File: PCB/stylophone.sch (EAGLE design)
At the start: 24 parts, among them IC2 LM358N

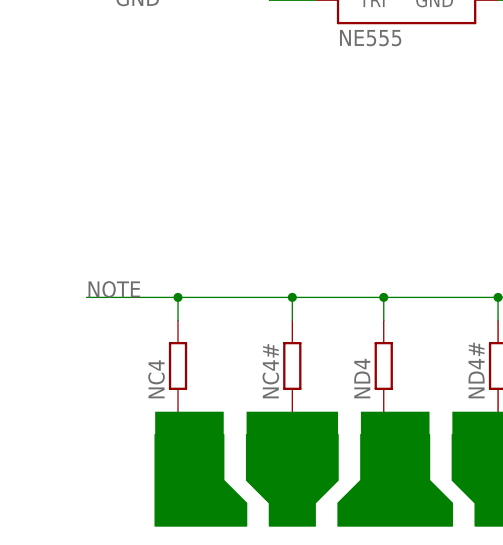
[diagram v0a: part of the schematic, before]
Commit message: almost done
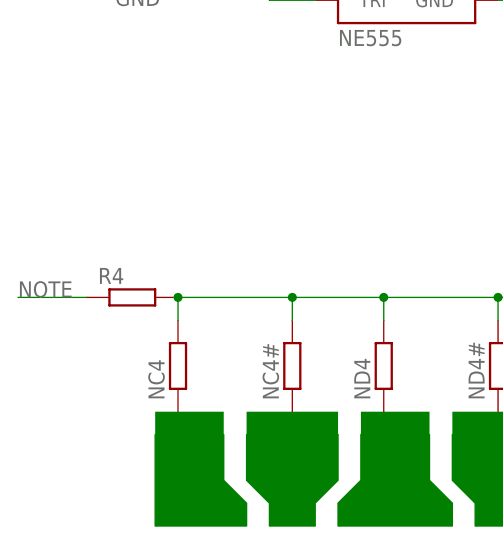
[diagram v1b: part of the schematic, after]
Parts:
- added R4: (no value), rcl:R-EU_0204/5
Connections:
- new net KEYBOARD: NA4#.2, NA4.2, NB4.2, NC4#.2, NC4.2, ND4#.2, ND4.2, NE4.2, NF4#.2, NF4.2, NG4#.2, NG4.2, R4.2
- net NOTE: now also R4.1; no longer NA4#.2, NA4.2, NB4.2, NC4#.2, NC4.2, ND4#.2, ND4.2, NE4.2, NF4#.2, NF4.2, NG4#.2, NG4.2
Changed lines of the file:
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@@
 <part name="R8" library="resistor" deviceset="R-TRIMM" device="5X"/>
 <part name="SV2" library="con-lstb" deviceset="MA05-1" device=""/>
+<part name="R4" library="rcl" deviceset="R-EU_" device="0204/5"/>
 </parts>
 <sheets>
@@
 <instance part="R8" gate="G$1" x="142.24" y="127"/>
 <instance part="SV2" gate="G$1" x="226.06" y="127" rot="R180"/>
+<instance part="R4" gate="G$1" x="25.4" y="86.36"/>
 </instances>
 <busses>
@@
 </segment>
 <segment>
+<pinref part="R4" gate="G$1" pin="1"/>
+<wire x1="20.32" y1="86.36" x2="12.7" y2="86.36" width="0.1524" layer="91"/>
+<label x="12.7" y="86.36" size="1.778" layer="95"/>
+</segment>
+</net>
+<net name="N$1" class="0">
+<segment>
+<pinref part="VIBRATO" gate="G$1" pin="CON"/>
+<wire x1="134.62" y1="121.92" x2="137.16" y2="121.92" width="0.1524" layer="91"/>
+<pinref part="C4" gate="G$1" pin="1"/>
+<wire x1="137.16" y1="121.92" x2="139.7" y2="119.38" width="0.1524" layer="91"/>
+</segment>
+</net>
+<net name="N$3" class="0">
+<segment>
+<pinref part="R7" gate="G$1" pin="1"/>
+<pinref part="R3" gate="G$1" pin="2"/>
+<wire x1="111.76" y1="144.78" x2="119.38" y2="144.78" width="0.1524" layer="91"/>
+<pinref part="VIBRATO" gate="G$1" pin="DIS"/>
+<wire x1="114.3" y1="127" x2="111.76" y2="127" width="0.1524" layer="91"/>
+<wire x1="111.76" y1="127" x2="111.76" y2="144.78" width="0.1524" layer="91"/>
+<junction x="111.76" y="144.78"/>
+</segment>
+</net>
+<net name="NOTSTYLUS" class="0">
+<segment>
+<pinref part="VIBRATO" gate="G$1" pin="TRI"/>
+<wire x1="114.3" y1="119.38" x2="109.22" y2="119.38" width="0.1524" layer="91"/>
+<wire x1="109.22" y1="119.38" x2="109.22" y2="134.62" width="0.1524" layer="91"/>
+<pinref part="VIBRATO" gate="G$1" pin="TRE"/>
+<wire x1="109.22" y1="134.62" x2="114.3" y2="134.62" width="0.1524" layer="91"/>
+<pinref part="C3" gate="G$1" pin="1"/>
+<wire x1="109.22" y1="134.62" x2="101.6" y2="134.62" width="0.1524" layer="91"/>
+<junction x="109.22" y="134.62"/>
+<pinref part="R7" gate="G$1" pin="2"/>
+<wire x1="101.6" y1="134.62" x2="99.06" y2="134.62" width="0.1524" layer="91"/>
+<wire x1="101.6" y1="144.78" x2="101.6" y2="134.62" width="0.1524" layer="91"/>
+<junction x="101.6" y="134.62"/>
+</segment>
+</net>
+<net name="N$2" class="0">
+<segment>
+<pinref part="VIBRATO" gate="G$1" pin="OUT"/>
+<wire x1="134.62" y1="127" x2="139.7" y2="132.08" width="0.1524" layer="91"/>
+<pinref part="R8" gate="G$1" pin="A"/>
+<wire x1="139.7" y1="132.08" x2="142.24" y2="132.08" width="0.1524" layer="91"/>
+</segment>
+</net>
+<net name="N$5" class="0">
+<segment>
+<pinref part="R1" gate="G$1" pin="S"/>
+<pinref part="IC2" gate="A" pin="+IN"/>
+<wire x1="182.88" y1="127" x2="185.42" y2="127" width="0.1524" layer="91"/>
+</segment>
+</net>
+<net name="KEYBOARD" class="0">
+<segment>
 <pinref part="NB4" gate="G$1" pin="2"/>
 <wire x1="157.48" y1="83.82" x2="154.94" y2="86.36" width="0.1524" layer="91"/>
-<label x="20.32" y="86.36" size="1.778" layer="95"/>
 <pinref part="NA4#" gate="G$1" pin="2"/>
 <wire x1="144.78" y1="83.82" x2="144.78" y2="86.36" width="0.1524" layer="91"/>
@@
 <wire x1="43.18" y1="86.36" x2="30.48" y2="86.36" width="0.1524" layer="91"/>
 <junction x="43.18" y="86.36"/>
-<wire x1="30.48" y1="86.36" x2="20.32" y2="86.36" width="0.1524" layer="91"/>
+<pinref part="R4" gate="G$1" pin="2"/>
 <junction x="30.48" y="86.36"/>
 </segment>
 </net>
-<net name="N$1" class="0">
-<segment>
-<pinref part="VIBRATO" gate="G$1" pin="CON"/>
-<wire x1="134.62" y1="121.92" x2="137.16" y2="121.92" width="0.1524" layer="91"/>
-<pinref part="C4" gate="G$1" pin="1"/>
-<wire x1="137.16" y1="121.92" x2="139.7" y2="119.38" width="0.1524" layer="91"/>
-</segment>
-</net>
-<net name="N$3" class="0">
-<segment>
-<pinref part="R7" gate="G$1" pin="1"/>
-<pinref part="R3" gate="G$1" pin="2"/>
-<wire x1="111.76" y1="144.78" x2="119.38" y2="144.78" width="0.1524" layer="91"/>
-<pinref part="VIBRATO" gate="G$1" pin="DIS"/>
-<wire x1="114.3" y1="127" x2="111.76" y2="127" width="0.1524" layer="91"/>
-<wire x1="111.76" y1="127" x2="111.76" y2="144.78" width="0.1524" layer="91"/>
-<junction x="111.76" y="144.78"/>
-</segment>
-</net>
-<net name="NOTSTYLUS" class="0">
-<segment>
-<pinref part="VIBRATO" gate="G$1" pin="TRI"/>
-<wire x1="114.3" y1="119.38" x2="109.22" y2="119.38" width="0.1524" layer="91"/>
-<wire x1="109.22" y1="119.38" x2="109.22" y2="134.62" width="0.1524" layer="91"/>
-<pinref part="VIBRATO" gate="G$1" pin="TRE"/>
-<wire x1="109.22" y1="134.62" x2="114.3" y2="134.62" width="0.1524" layer="91"/>
-<pinref part="C3" gate="G$1" pin="1"/>
-<wire x1="109.22" y1="134.62" x2="101.6" y2="134.62" width="0.1524" layer="91"/>
-<junction x="109.22" y="134.62"/>
-<pinref part="R7" gate="G$1" pin="2"/>
-<wire x1="101.6" y1="134.62" x2="99.06" y2="134.62" width="0.1524" layer="91"/>
-<wire x1="101.6" y1="144.78" x2="101.6" y2="134.62" width="0.1524" layer="91"/>
-<junction x="101.6" y="134.62"/>
-</segment>
-</net>
-<net name="N$2" class="0">
-<segment>
-<pinref part="VIBRATO" gate="G$1" pin="OUT"/>
-<wire x1="134.62" y1="127" x2="139.7" y2="132.08" width="0.1524" layer="91"/>
-<pinref part="R8" gate="G$1" pin="A"/>
-<wire x1="139.7" y1="132.08" x2="142.24" y2="132.08" width="0.1524" layer="91"/>
-</segment>
-</net>
-<net name="N$5" class="0">
-<segment>
-<pinref part="R1" gate="G$1" pin="S"/>
-<pinref part="IC2" gate="A" pin="+IN"/>
-<wire x1="182.88" y1="127" x2="185.42" y2="127" width="0.1524" layer="91"/>
-</segment>
-</net>
